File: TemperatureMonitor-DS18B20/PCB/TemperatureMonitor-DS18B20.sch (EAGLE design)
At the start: 13 parts, among them IC1 ESP8266MINI, IC2 MCP1700 3300, IC3 SSD1306, SW1 SensorID, SW2 DeepSleep, T1 DS18B20

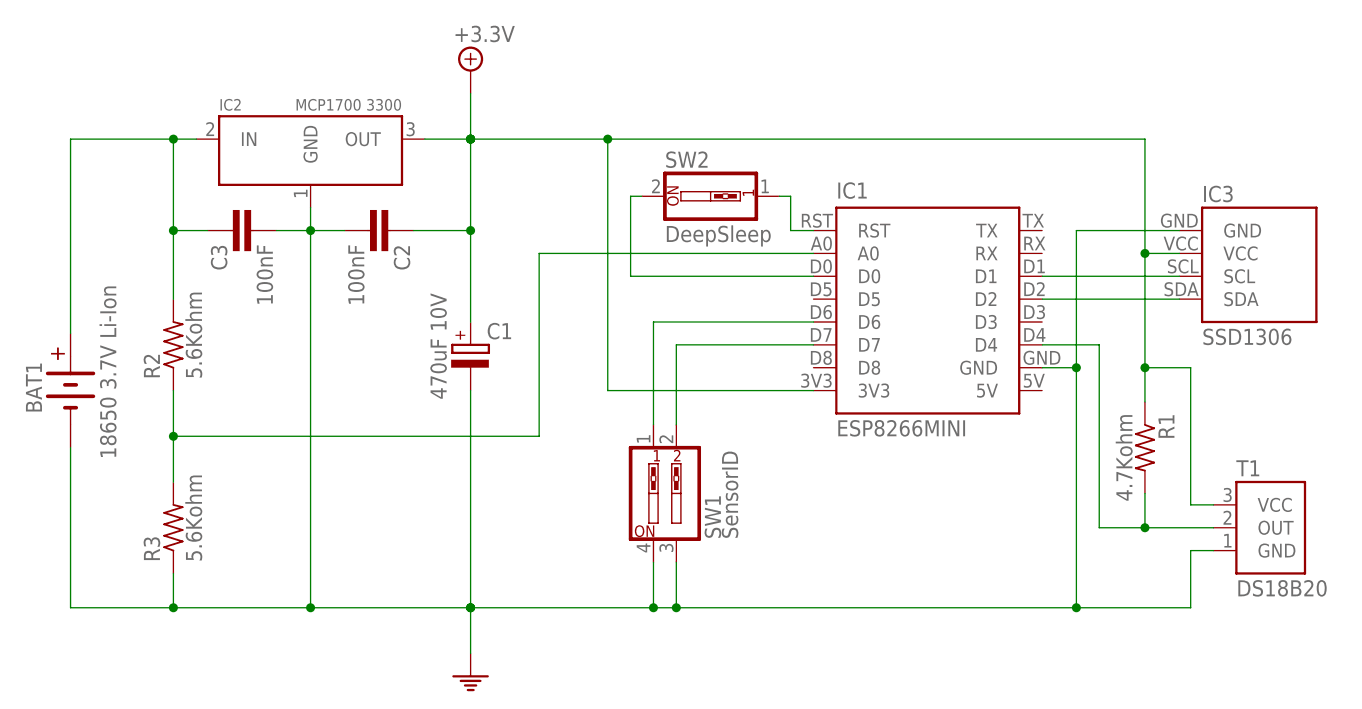
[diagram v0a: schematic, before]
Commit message: Minor changes
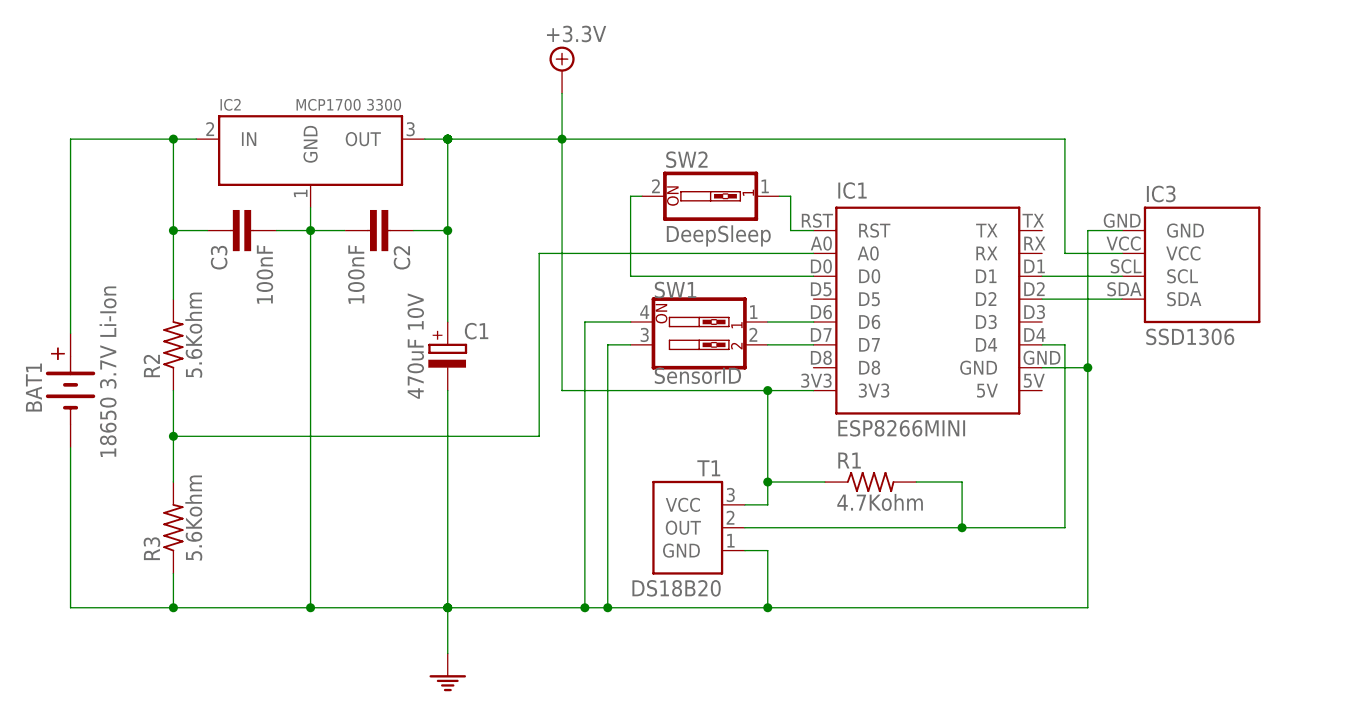
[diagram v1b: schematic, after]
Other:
- moved on the sheet: C1, IC3, R1, SW1, T1
